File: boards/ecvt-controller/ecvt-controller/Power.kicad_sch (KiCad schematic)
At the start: 6 parts, among them Q1 Q_PMOS_GDS

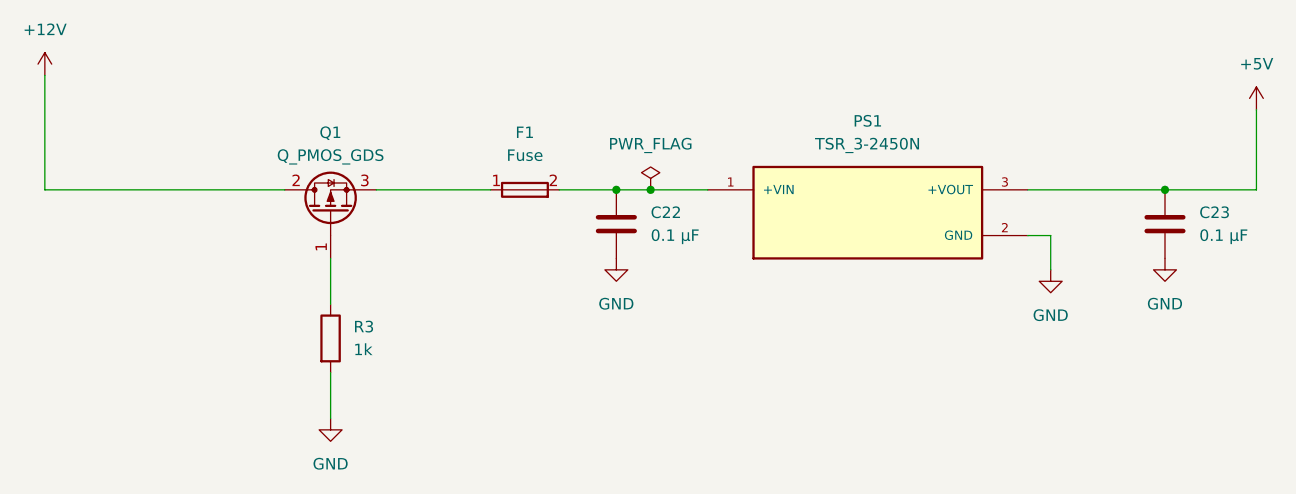
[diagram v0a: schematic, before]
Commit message: can you CANCAN
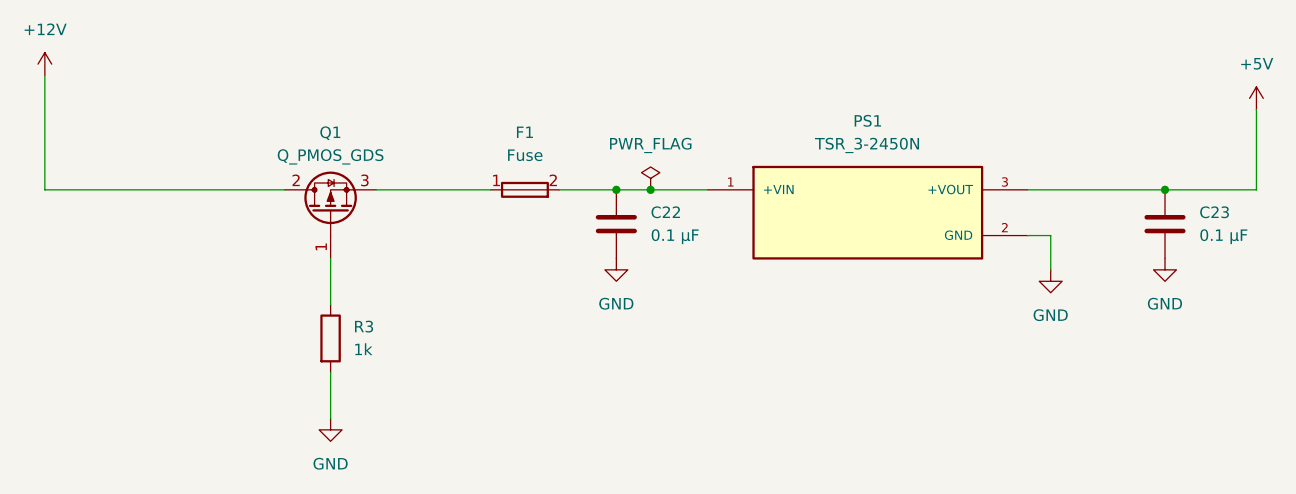
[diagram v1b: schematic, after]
